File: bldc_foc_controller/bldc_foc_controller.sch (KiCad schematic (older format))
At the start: 155 parts

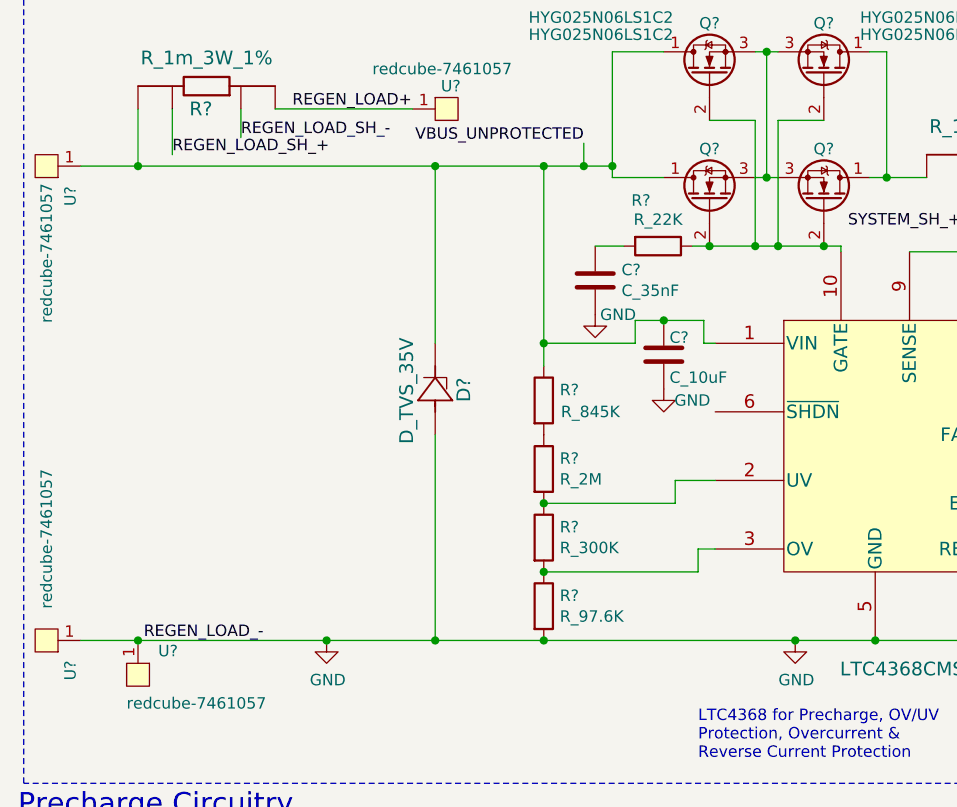
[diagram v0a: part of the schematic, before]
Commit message: simple changes yuh
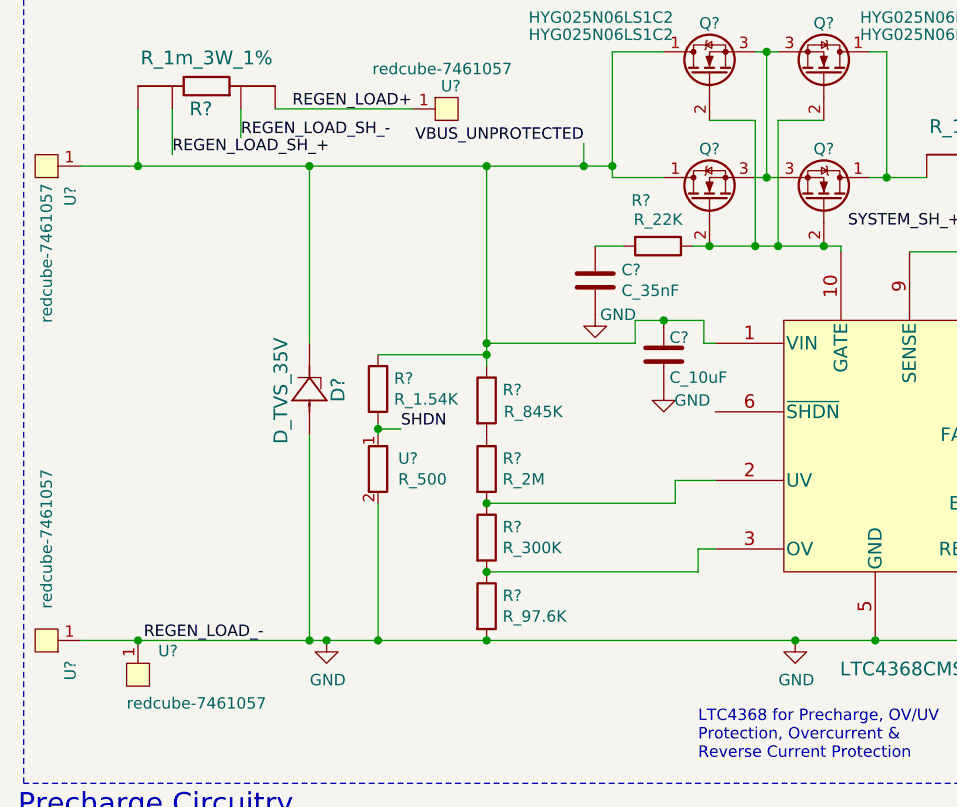
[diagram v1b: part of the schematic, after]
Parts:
- added R?: R_1.54K, footprints:R_0805_OEM, symbol formula:R_1.54K
- added U?: R_500, footprints:R_0805_OEM, symbol formula:R_500
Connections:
- net GND: now also U?.2
- net VBUS_UNPROTECTED: now also R?.1
- new net SHDN: R?.2, U?.1
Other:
- moved on the sheet: D?, R?
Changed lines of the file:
@@
 	1    0    0    -1
 $EndComp
-Connection ~ 3950 3500
 $Comp
 L power:+10V #PWR0109
@@
 L Device:R R?
 U 1 1 61B4CA23
-P 2850 2450
-F 0 "R?" H 2920 2496 50  0000 L CNN
-F 1 "R_845K" H 2925 2400 50  0000 L CNN
-F 2 "footprints:R_0805_OEM" V 2780 2450 50  0001 C CNN
-F 3 "https://www.digikey.com/en/products/detail/stackpole-electronics-inc/RMCF0805FT845K/1713403" H 2850 2450 50  0001 C CNN
-	1    2850 2450
+P 2600 2450
+F 0 "R?" H 2670 2496 50  0000 L CNN
+F 1 "R_845K" H 2675 2400 50  0000 L CNN
+F 2 "footprints:R_0805_OEM" V 2530 2450 50  0001 C CNN
+F 3 "https://www.digikey.com/en/products/detail/stackpole-electronics-inc/RMCF0805FT845K/1713403" H 2600 2450 50  0001 C CNN
+	1    2600 2450
 	1    0    0    -1
 $EndComp
@@
 L Device:R R?
 U 1 1 61B5D3A0
-P 2850 2750
-F 0 "R?" H 2920 2796 50  0000 L CNN
-F 1 "R_2M" H 2920 2705 50  0000 L CNN
-F 2 "footprints:R_0805_OEM" V 2780 2750 50  0001 C CNN
-F 3 "https://www.digikey.com/en/products/detail/stackpole-electronics-inc/RMCF0805FT2M00/1760219" H 2850 2750 50  0001 C CNN
-	1    2850 2750
+P 2600 2750
+F 0 "R?" H 2670 2796 50  0000 L CNN
+F 1 "R_2M" H 2670 2705 50  0000 L CNN
+F 2 "footprints:R_0805_OEM" V 2530 2750 50  0001 C CNN
+F 3 "https://www.digikey.com/en/products/detail/stackpole-electronics-inc/RMCF0805FT2M00/1760219" H 2600 2750 50  0001 C CNN
+	1    2600 2750
 	1    0    0    -1
 $EndComp
@@
 Connection ~ 1075 3500
 Wire Wire Line
-	1075 3500 1900 3500
+	1075 3500 1825 3500
 Text Label 1100 3500 0    50   ~ 0
 REGEN_LOAD_-
@@
 Text Label 4225 10050 0    50   ~ 0
 SNS_SH_SYSTEM
-Connection ~ 2850 1425
-Wire Wire Line
-	2850 1425 3025 1425
 $Comp
 L formula:R_300K R?
 U 1 1 692D0260
-P 2850 3050
-F 0 "R?" H 2920 3096 50  0000 L CNN
-F 1 "R_300K" H 2920 3005 50  0000 L CNN
-F 2 "footprints:R_0805_OEM" H 2780 3050 50  0001 C CNN
-F 3 "https://industrial.panasonic.com/cdbs/www-data/pdf/RDM0000/AOA0000C307.pdf" H 2930 3050 50  0001 C CNN
-F 4 "DK" H 2850 3050 60  0001 C CNN "MFN"
-F 5 "P300KDACT-ND" H 2850 3050 60  0001 C CNN "MPN"
-F 6 "https://www.digikey.com/product-detail/en/panasonic-electronic-components/ERA-6AEB304V/P300KDACT-ND/1466006" H 3330 3450 60  0001 C CNN "PurchasingLink"
-	1    2850 3050
+P 2600 3050
+F 0 "R?" H 2670 3096 50  0000 L CNN
+F 1 "R_300K" H 2670 3005 50  0000 L CNN
+F 2 "footprints:R_0805_OEM" H 2530 3050 50  0001 C CNN
+F 3 "https://industrial.panasonic.com/cdbs/www-data/pdf/RDM0000/AOA0000C307.pdf" H 2680 3050 50  0001 C CNN
+F 4 "DK" H 2600 3050 60  0001 C CNN "MFN"
+F 5 "P300KDACT-ND" H 2600 3050 60  0001 C CNN "MPN"
+F 6 "https://www.digikey.com/product-detail/en/panasonic-electronic-components/ERA-6AEB304V/P300KDACT-ND/1466006" H 3080 3450 60  0001 C CNN "PurchasingLink"
+	1    2600 3050
 	1    0    0    -1
 $EndComp
@@
 L Device:R R?
 U 1 1 693C1FA4
-P 2850 3350
-F 0 "R?" H 2920 3396 50  0000 L CNN
-F 1 "R_97.6K" H 2920 3305 50  0000 L CNN
-F 2 "footprints:R_0805_OEM" V 2780 3350 50  0001 C CNN
-F 3 "~" H 2850 3350 50  0001 C CNN
-	1    2850 3350
+P 2600 3350
+F 0 "R?" H 2670 3396 50  0000 L CNN
+F 1 "R_97.6K" H 2670 3305 50  0000 L CNN
+F 2 "footprints:R_0805_OEM" V 2530 3350 50  0001 C CNN
+F 3 "~" H 2600 3350 50  0001 C CNN
+	1    2600 3350
 	1    0    0    -1
 $EndComp
-Connection ~ 2850 3500
+Connection ~ 2600 3500
 Wire Wire Line
 	3525 3100 3525 3200
 Wire Wire Line
-	3250 2200 2850 2200
-Wire Wire Line
-	2850 1425 2850 2200
-Connection ~ 2850 2200
+	2600 1425 2600 2200
+Connection ~ 2600 2200
 Wire Wire Line
 	3550 2200 3600 2200
@@
 $Comp
 L formula:D_TVS_35V D?
-U 1 1 61F5EEBD
-P 2375 2600
-F 0 "D?" H 2625 2475 60  0000 R CNN
-F 1 "D_TVS_35V" H 2800 2725 60  0000 R CNN
-F 2 "SMC_DIO" H 2575 2240 60  0001 C CNN
-F 3 "https://www.diodes.com/assets/Datasheets/ds40741.pdf" H 2375 2600 60  0001 C CNN
-F 4 "SMCJ22A-13-F" H 2525 2850 50  0001 C CNN "MPN"
-	1    2375 2600
-	0    -1   -1   0
-$EndComp
-$Comp
-L formula:D_TVS_35V D?
 U 1 1 61FF9FF0
 P 5850 2450
@@
 	0    -1   -1   0
 $EndComp
-Wire Wire Line
-	2375 2600 2375 3500
-Wire Wire Line
-	2375 3500 2850 3500
-Wire Wire Line
-	2375 2200 2375 1425
-Wire Wire Line
-	1075 1425 2375 1425
-Connection ~ 2375 1425
-Wire Wire Line
-	2375 1425 2850 1425
 $Comp
 L Mechanical:MountingHole_Pad H?
@@
 Wire Wire Line
 	9250 7700 9425 7700
-Connection ~ 2850 2900
-Connection ~ 2850 3200
-Wire Wire Line
-	2850 2900 3425 2900
-Wire Wire Line
-	2850 3200 3525 3200
-Connection ~ 2375 3500
+Connection ~ 2600 2900
+Connection ~ 2600 3200
 Wire Wire Line
 	3425 2900 3425 2800
 Wire Wire Line
-	1900 3500 2375 3500
-Wire Wire Line
-	2850 3500 3950 3500
-Wire Wire Line
-	2850 2200 2850 2300
+	2600 2200 2600 2250
 Connection ~ 1775 5025
 $Comp
@@
 	1    0    0    -1
 $EndComp
+Connection ~ 2600 1425
+Wire Wire Line
+	2600 1425 3025 1425
+Wire Wire Line
+	2600 2900 3425 2900
+Wire Wire Line
+	2600 3200 3525 3200
+Wire Wire Line
+	2600 3500 3950 3500
+Connection ~ 3950 3500
+Wire Wire Line
+	2600 2200 3250 2200
+Wire Wire Line
+	1075 1425 1825 1425
+Wire Wire Line
+	1825 2200 1825 1425
+Wire Wire Line
+	1825 2600 1825 3500
+$Comp
+L formula:D_TVS_35V D?
+U 1 1 61F5EEBD
+P 1825 2600
+F 0 "D?" H 2075 2475 60  0000 R CNN
+F 1 "D_TVS_35V" H 2250 2725 60  0000 R CNN
+F 2 "SMC_DIO" H 2025 2240 60  0001 C CNN
+F 3 "https://www.diodes.com/assets/Datasheets/ds40741.pdf" H 1825 2600 60  0001 C CNN
+F 4 "SMCJ22A-13-F" H 1975 2850 50  0001 C CNN "MPN"
+	1    1825 2600
+	0    -1   -1   0
+$EndComp
+$Comp
+L formula:R_1.54K R?
+U 1 1 61D037A0
+P 2125 2400
+F 0 "R?" H 2195 2446 50  0000 L CNN
+F 1 "R_1.54K" H 2195 2355 50  0000 L CNN
+F 2 "footprints:R_0805_OEM" H 2055 2400 50  0001 C CNN
+F 3 "https://industrial.panasonic.com/cdbs/www-data/pdf/RDA0000/AOA0000C304.pdf" H 2205 2400 50  0001 C CNN
+F 4 "Panasonic" H 2125 2400 50  0001 C CNN "MFN"
+F 5 "ERJ-6ENF1541V" H 2125 2400 50  0001 C CNN "MPN"
+F 6 "https://www.digikey.com/en/products/detail/panasonic-electronic-components/ERJ-6ENF1541V/111317" H 2125 2400 50  0001 C CNN "Purchasing Link"
+	1    2125 2400
+	1    0    0    -1
+$EndComp
+$Comp
+L formula:R_500 U?
+U 1 1 61D01F28
+P 2125 2750
+F 0 "U?" V 2079 2838 50  0000 L CNN
+F 1 "R_500" V 2170 2838 50  0000 L CNN
+F 2 "footprints:R_0805_OEM" H 2125 2750 50  0001 C CNN
+F 3 "" H 2125 2750 50  0001 C CNN
+	1    2125 2750
+	0    1    1    0
+$EndComp
+Connection ~ 1825 1425
+Connection ~ 1825 3500
+Wire Wire Line
+	1825 3500 1900 3500
+Wire Wire Line
+	1825 1425 2600 1425
+Wire Wire Line
+	2125 2550 2125 2575
+Wire Wire Line
+	2125 2250 2600 2250
+Connection ~ 2600 2250
+Wire Wire Line
+	2600 2250 2600 2300
+Wire Wire Line
+	2125 2900 2125 3500
+Wire Wire Line
+	1900 3500 2125 3500
+Connection ~ 2125 3500
+Wire Wire Line
+	2125 3500 2600 3500
+Wire Wire Line
+	2125 2575 2225 2575
+Connection ~ 2125 2575
+Wire Wire Line
+	2125 2575 2125 2600
+Text Label 2225 2575 0    50   ~ 0
+SHDN
 $EndSCHEMATC
